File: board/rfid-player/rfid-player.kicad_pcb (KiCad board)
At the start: 2 copper layers, 106.4 x 77.2 mm, 22 parts

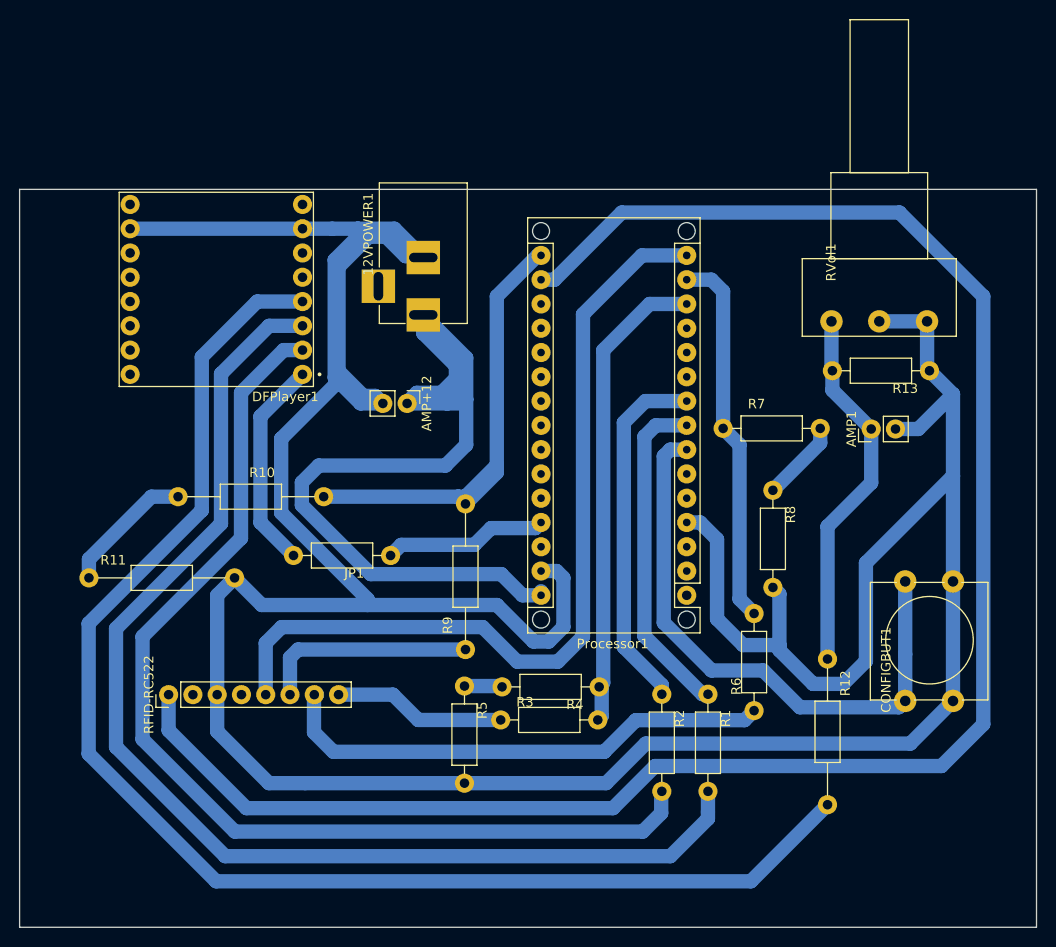
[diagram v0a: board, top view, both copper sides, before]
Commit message: Board fixes
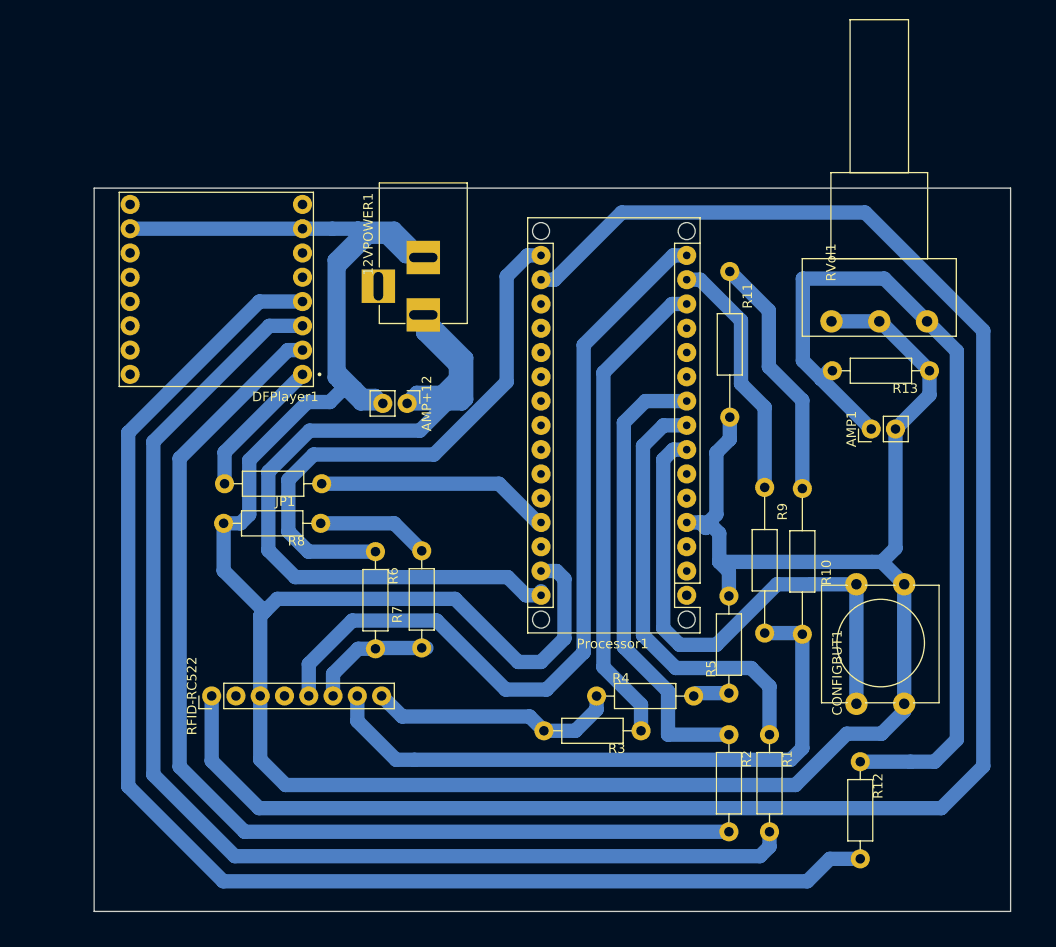
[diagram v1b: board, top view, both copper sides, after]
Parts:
- R10, R3, R4, R6, R7, R9: value R -> 2k2
- R11, R5, R8: value R -> 1k
- R12: footprint Resistors_THT:R_Axial_DIN0207_L6.3mm_D2.5mm_P15.24mm_Horizontal -> Resistors_THT:R_Axial_DIN0207_L6.3mm_D2.5mm_P10.16mm_Horizontal
- moved R11 74.3 mm to (91.8, 24.8), turned to 270 degrees
- moved R10 52.1 mm to (99.4, 62.8), turned to 90 degrees
- moved R8 47.4 mm to (49.0, 51.2), turned to 180 degrees
- moved R6 43.0 mm to (54.7, 54.1), turned to 270 degrees
- moved R7 39.0 mm to (59.6, 64.2), turned to 90 degrees
- moved R9 35.6 mm to (95.4, 47.4), turned to 270 degrees
- moved R5 27.7 mm to (91.7, 68.9), turned to 90 degrees
- moved R3 14.7 mm to (82.5, 72.9), turned to 180 degrees
- moved R12 11.3 mm to (105.4, 76.1)
- moved JP1 10.4 mm to (49.1, 47.0)
- moved R2 8.20 mm to (91.7, 73.3)
- moved R1 7.70 mm to (95.9, 73.3)
- moved CONFIGBUT1 5.11 mm to (105.0, 70.0)
- moved RFID-RC522 4.51 mm to (37.6, 69.2)
- moved R4 0.99 mm to (77.9, 69.2), turned to 0 degrees
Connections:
- R10 pad 1: D13 -> SCK
- R3 pad 1: SDA -> D10
- R3 pad 2: D10 -> SDA
- R4 pad 1: D10 -> SDA
- R6 pad 1: SCK -> D13
- R6 pad 2: D11 -> MOSI
- R7 pad 1: D11 -> MOSI
- R9 pad 1: MOSI -> D11
- R9 pad 2: D13 -> SCK
- RVol1 pad 1: GND -> Net-(AMP1-Pad1)
- RVol1 pad 3: Net-(AMP1-Pad1) -> GND
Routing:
- net Net-(AMP1-Pad1): track 38.9 -> 91.6 mm
- net GND: track 373.9 -> 341.6 mm
- net SCK: track 53.0 -> 67.3 mm
- net D11: track 39.4 -> 25.9 mm
- net Net-(R10-Pad2): track 14.0 -> 25.9 mm
- net Net-(Processor1-Pad9): track 37.6 -> 48.4 mm
- net Net-(Processor1-Pad8): track 34.9 -> 45.8 mm
- net MOSI: track 22.6 -> 13.2 mm
- net SDA: track 18.1 -> 26.3 mm
- net D13: track 50.0 -> 58.0 mm
- net Net-(JP1-Pad1): track 17.2 -> 24.6 mm
- net 5V: track 22.2 -> 14.8 mm
- net 12V: track 89.7 -> 95.1 mm
- net Net-(CONFIGBUT1-Pad1): track 61.8 -> 56.6 mm
- net MISO: track 89.0 -> 85.4 mm
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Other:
- board size 106.4 x 77.2 mm -> 95.9 x 75.7 mm
